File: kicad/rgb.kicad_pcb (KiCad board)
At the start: 2 copper layers, 25 parts, among them J1 1935776, J2 Conn_01x05, J3 Conn_01x05, J4 Conn_01x04, J5 Conn_01x02, Q1 DMG9926USD, Q2 DMG9926USD, Q3 DMG9926USD, Q4 DMG9926USD, SW1 SW_Push, SW2 Rotary_Encoder, SW3 Rotary_Encoder, SW4 Rotary_Encoder, SW5 Rotary_Encoder, SW6 SW_Push, U1 ATtiny416-SNR, U2 MIC5203

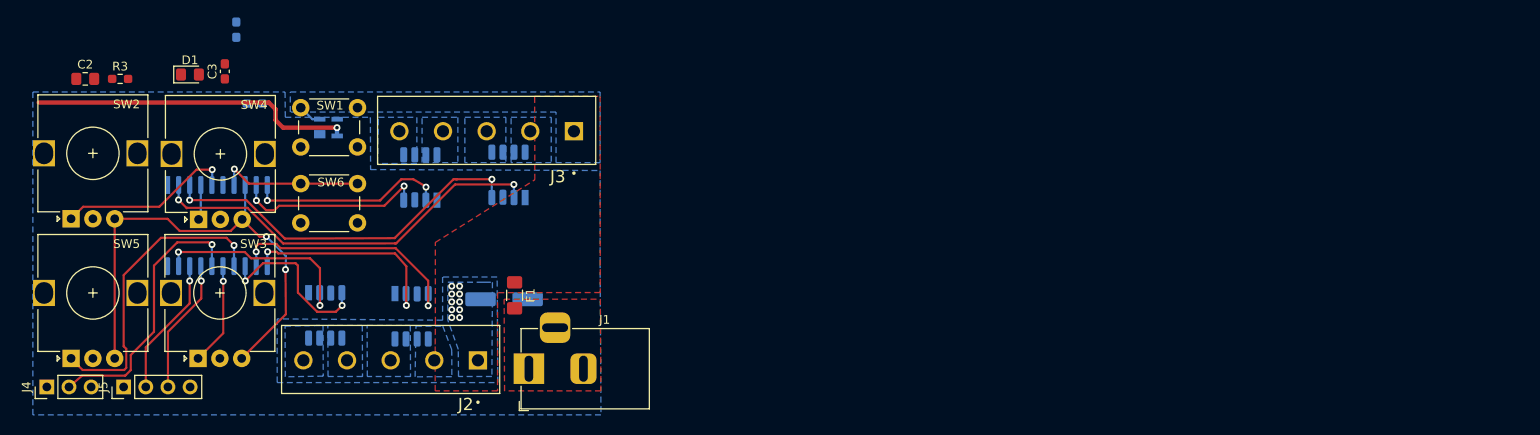
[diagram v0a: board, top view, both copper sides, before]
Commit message: pcb layout + mounting
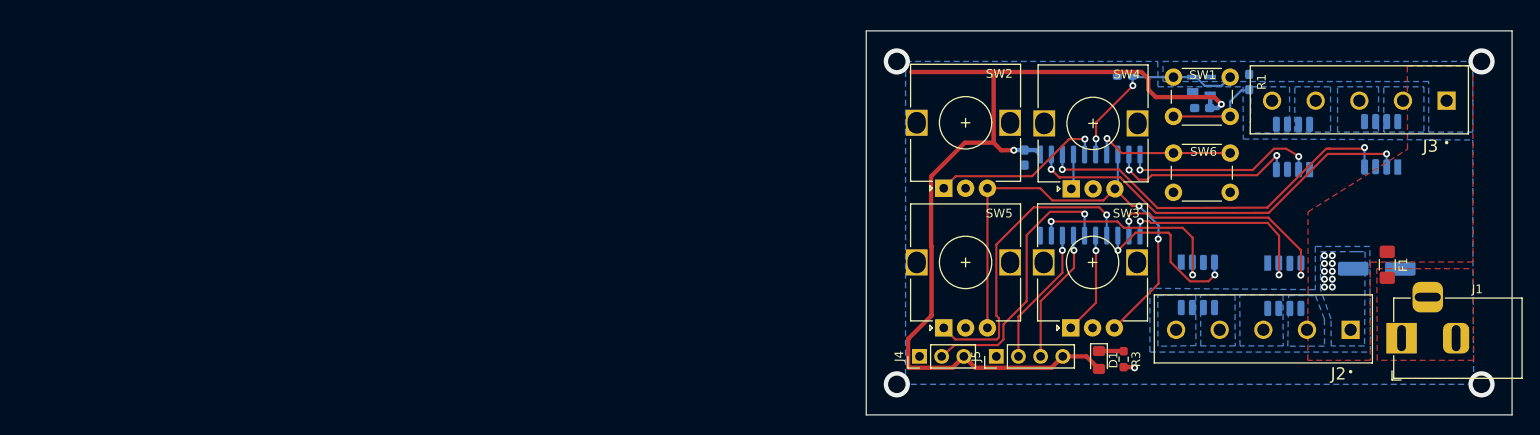
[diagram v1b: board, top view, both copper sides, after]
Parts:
- C2: footprint Capacitor_SMD:C_0805_2012Metric_Pad1.15x1.40mm_HandSolder -> Capacitor_SMD:C_0603_1608Metric_Pad1.08x0.95mm_HandSolder; moved to B.Cu
- C3: moved to B.Cu
- moved C2 128.0 mm to (160.5, 65.8), turned to 180 degrees
- moved R3 119.4 mm to (151.5, 94.6), turned to 270 degrees
- moved R1 114.0 mm to (165.9, 62.9), turned to 90 degrees
- moved D1 109.2 mm to (148.7, 94.7), turned to 270 degrees
- moved R2 102.0 mm to (151.6, 62.1), turned to 180 degrees
- moved U2 100.2 mm to (160.4, 63.3)
- moved C1 100.1 mm to (180.5, 84.2)
- moved J1 100.1 mm to (188.8, 83.8)
- moved J2 100.1 mm to (177.5, 91.2)
- moved J3 100.1 mm to (188.5, 65.0)
- moved J4 100.1 mm to (128.1, 94.3)
- moved J5 100.1 mm to (136.9, 94.3)
- moved Q1 100.1 mm to (169.9, 86.2)
- moved Q2 100.1 mm to (160.0, 86.1)
- moved Q3 100.1 mm to (181.0, 70.0)
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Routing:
- net +5V: track 37.1 -> 110.8 mm, vias 1 -> 2
- net /PWR_EN: track 2.72 -> 23.0 mm, vias 0 -> 2
- net Net-(R1-Pad1): track 0.62 -> 11.5 mm
- net Net-(D1-Pad1): track 0.00 -> 2.84 mm
- net GND: track 0.00 -> 1.29 mm, vias 0 -> 1
- net (no net): vias 0 -> 4
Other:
- board outline added: 74 x 44 mm
